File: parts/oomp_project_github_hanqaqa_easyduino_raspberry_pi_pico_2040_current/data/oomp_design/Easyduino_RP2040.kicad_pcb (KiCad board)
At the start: 4 copper layers, 21 x 51 mm, 65 parts, among them J1 USB_C_Receptacle_USB2.0, J3 Conn_01x20, J4 Conn_01x20, J5 Conn_01x03, J6 Conn_01x03_MountingPin, SW1 SW_Push, SW2 SW_Push, U1 XC6206P332MR, U2 RP2040, U3 W25Q16JVUXIQ, Y1 12MHz

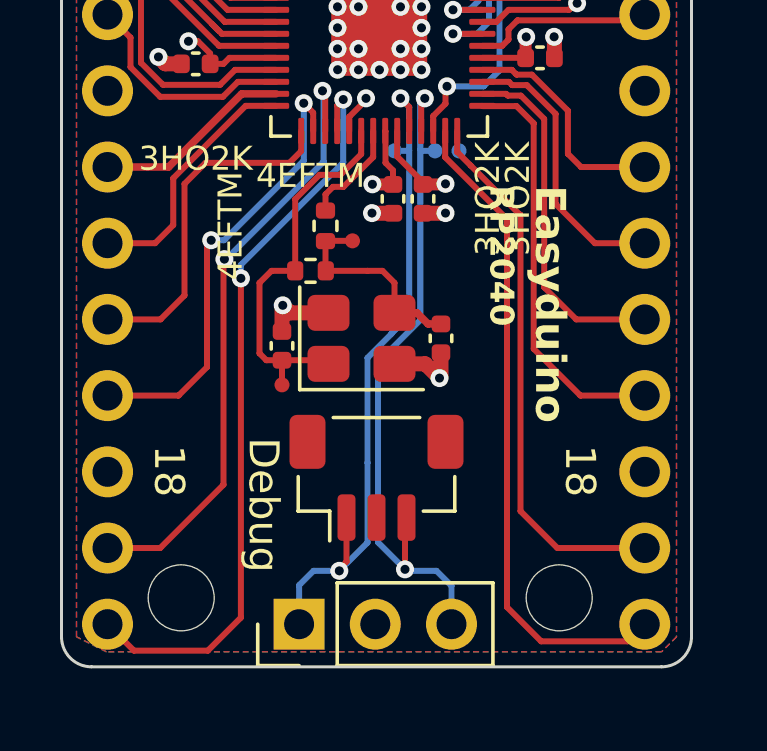
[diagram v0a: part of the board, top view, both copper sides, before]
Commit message: changes
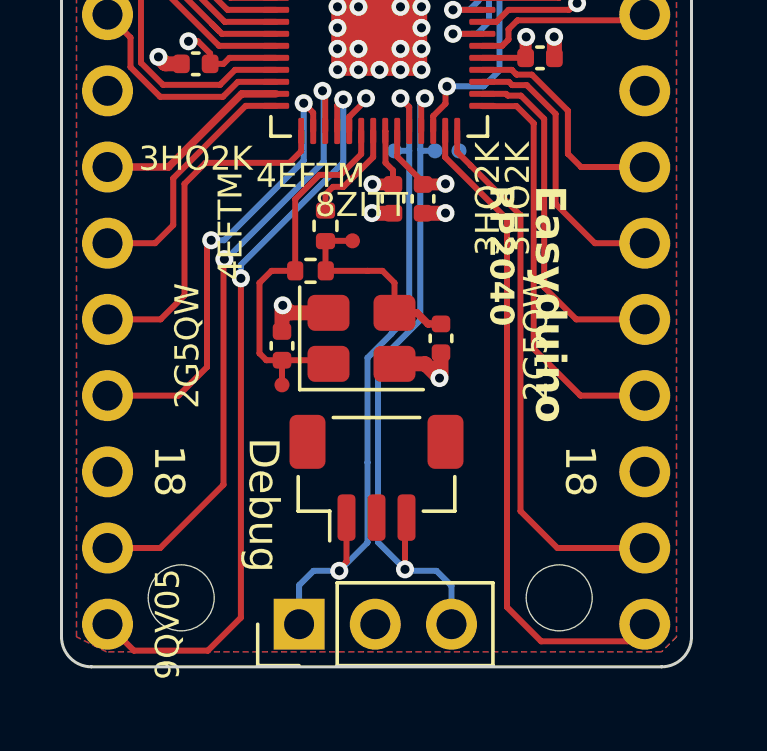
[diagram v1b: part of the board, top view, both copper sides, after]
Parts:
- C16, C17: footprint Capacitor_SMD:C_0402_1005Metric -> OOMP_MachineSolder:electronic_capacitor_0402_27_pico_farad
- J5: footprint Connector_PinHeader_2.54mm:PinHeader_1x03_P2.54mm_Vertical -> OOMP_MachineSolder:electronic_connector_header_2_54_mm_pitch_through_hole_3_pin
- Y1: footprint Crystal:Crystal_SMD_3225-4Pin_3.2x2.5mm -> OOMP_MachineSolder:electronic_crystal_3225_surface_mount_4_pin_12_mhz_20_pf

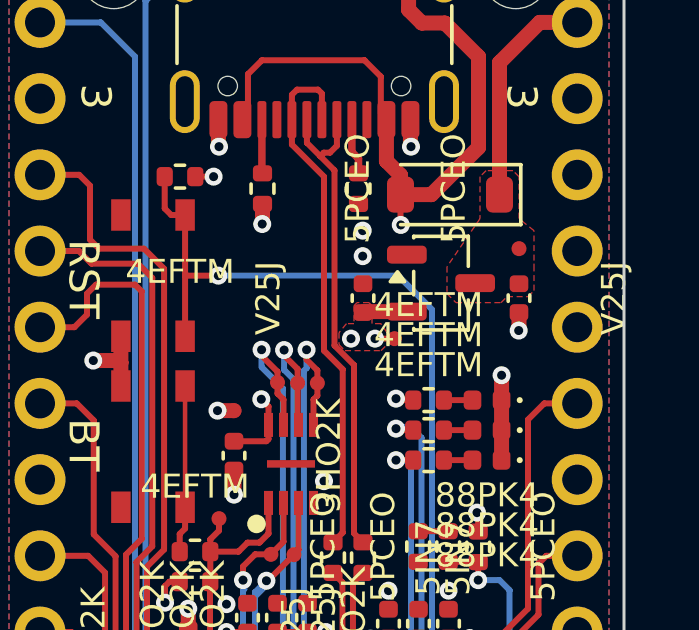
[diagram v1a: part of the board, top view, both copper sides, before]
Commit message: current
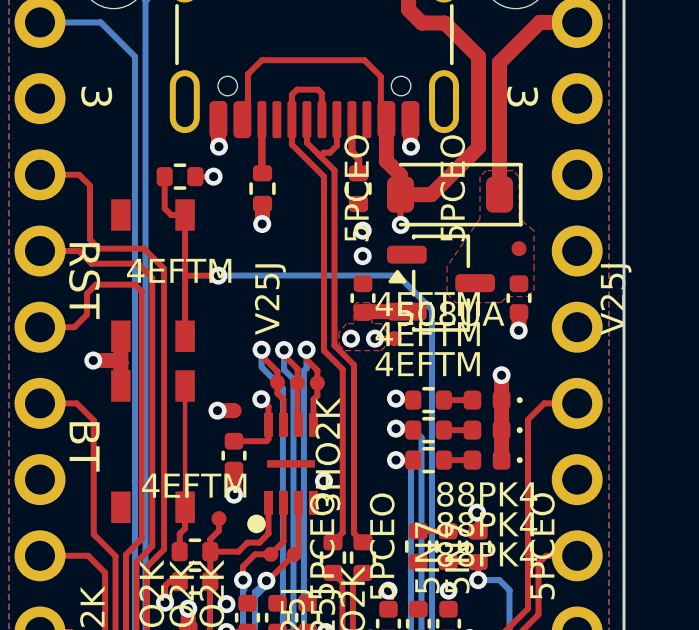
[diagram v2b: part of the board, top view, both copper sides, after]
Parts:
- D1: footprint Diode_SMD:D_SOD-123 -> OOMP_MachineSolder:electronic_diode_schottky_sod_123_ss14

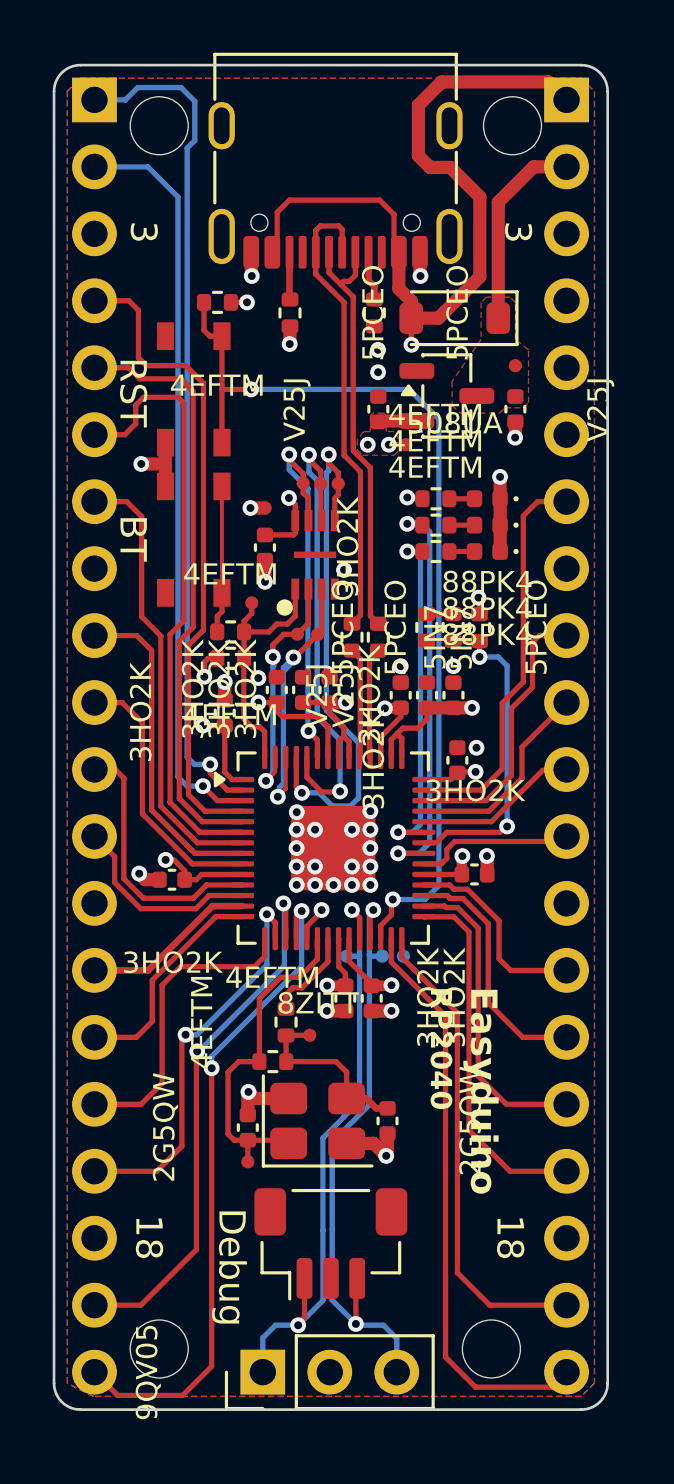
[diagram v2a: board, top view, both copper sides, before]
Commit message: working
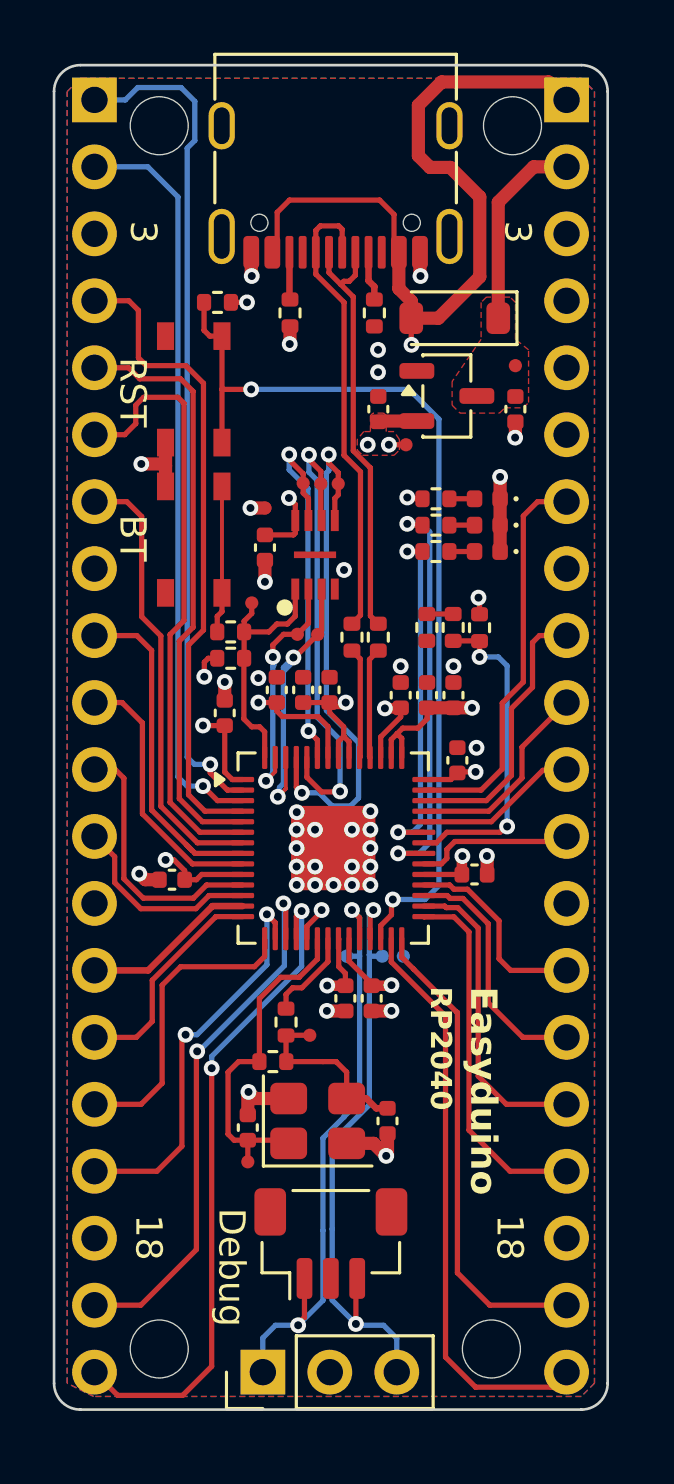
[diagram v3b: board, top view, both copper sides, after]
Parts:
- C1, C10, C11, C12, C15, C2, C5, C6, C7, C8, C9: footprint OOMP_MachineSolder:electronic_capacitor_0402_100_nano_farad -> Capacitor_SMD:C_0402_1005Metric
- C13, C14, C3, C4: footprint OOMP_MachineSolder:electronic_capacitor_0402_1_micro_farad -> Capacitor_SMD:C_0402_1005Metric
- C16, C17: footprint OOMP_MachineSolder:electronic_capacitor_0402_27_pico_farad -> Capacitor_SMD:C_0402_1005Metric
- D1: footprint OOMP_MachineSolder:electronic_diode_schottky_sod_123_ss14 -> Diode_SMD:D_SOD-123
- D2, D3, D4: footprint OOMP_MachineSolder:electronic_led_0402 -> LED_SMD:LED_0402_1005Metric
- J5: footprint OOMP_MachineSolder:electronic_connector_header_2_54_mm_pitch_through_hole_3_pin -> Connector_PinHeader_2.54mm:PinHeader_1x03_P2.54mm_Vertical
- R1, R2, R3, R6, R7: footprint OOMP_MachineSolder:electronic_resistor_0402_5100_ohm -> Resistor_SMD:R_0402_1005Metric
- R10, R11, R12, R13, R14, R15, R8, R9: footprint OOMP_MachineSolder:electronic_resistor_0402_1000_ohm -> Resistor_SMD:R_0402_1005Metric
- R4, R5: footprint OOMP_MachineSolder:electronic_resistor_0402_27_ohm -> Resistor_SMD:R_0402_1005Metric
- Y1: footprint OOMP_MachineSolder:electronic_crystal_3225_surface_mount_4_pin_12_mhz_20_pf -> Crystal:Crystal_SMD_3225-4Pin_3.2x2.5mm
